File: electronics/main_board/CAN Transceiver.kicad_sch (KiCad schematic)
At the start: 2 parts, among them U18 TJA1051TK/3

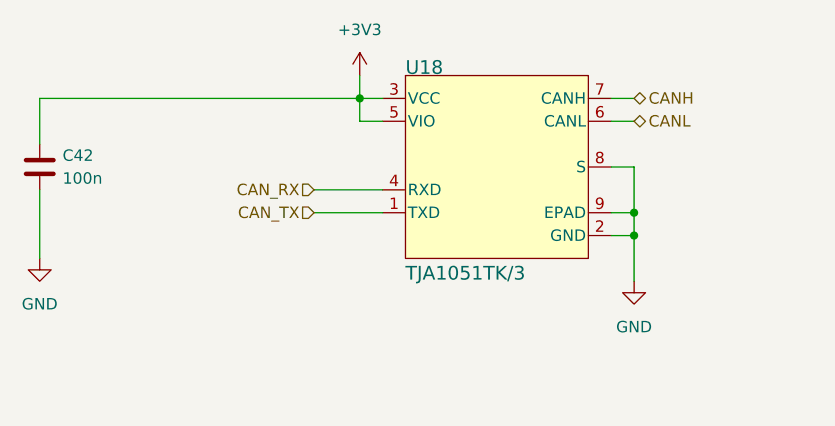
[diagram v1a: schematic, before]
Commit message: fix
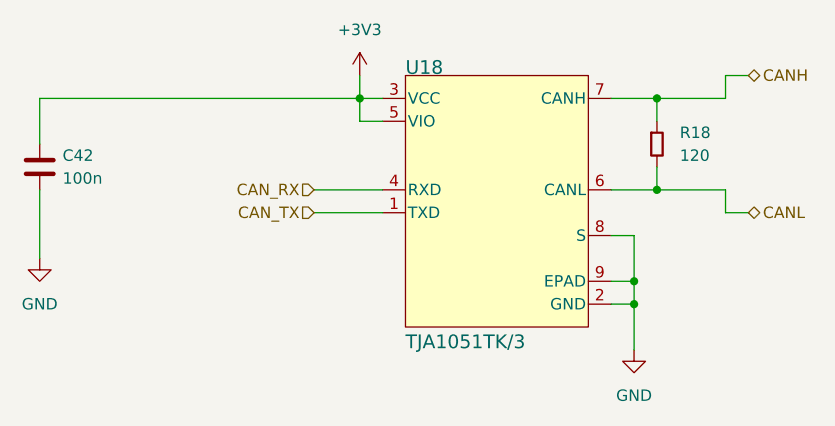
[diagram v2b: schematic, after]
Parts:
- added R18: 120, Resistor_SMD:R_0402_1005Metric, symbol Device:R
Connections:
- net CANH: now also R18.1
- net CANL: now also R18.2
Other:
- moved on the sheet: U18
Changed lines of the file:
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@@
 	(paper "A4")
 	(junction
-		(at 167.64 99.06)
+		(at 167.64 106.68)
+		(diameter 0)
+		(color 0 0 0 0)
+	)
+	(junction
+		(at 170.18 93.98)
 		(diameter 0)
 		(color 0 0 0 0)
@@
 	)
 	(junction
-		(at 167.64 96.52)
+		(at 170.18 83.82)
 		(diameter 0)
 		(color 0 0 0 0)
 	)
+	(junction
+		(at 167.64 104.14)
+		(diameter 0)
+		(color 0 0 0 0)
+	)
+	(wire
+		(pts
+			(xy 170.18 83.82) (xy 170.18 86.36)
+		)
+		(stroke
+			(width 0)
+			(type default)
+		)
+	)
 	(wire
 		(pts
@@
 	(wire
 		(pts
-			(xy 167.64 96.52) (xy 167.64 99.06)
+			(xy 177.8 81.28) (xy 177.8 83.82)
+		)
+		(stroke
+			(width 0)
+			(type default)
+		)
+	)
+	(wire
+		(pts
+			(xy 167.64 104.14) (xy 167.64 106.68)
 		)
 		(stroke
@@
 	(wire
 		(pts
+			(xy 165.1 93.98) (xy 170.18 93.98)
+		)
+		(stroke
+			(width 0)
+			(type default)
+		)
+	)
+	(wire
+		(pts
 			(xy 132.08 96.52) (xy 139.7 96.52)
 		)
@@
 	(wire
 		(pts
+			(xy 165.1 106.68) (xy 167.64 106.68)
+		)
+		(stroke
+			(width 0)
+			(type default)
+		)
+	)
+	(wire
+		(pts
+			(xy 177.8 96.52) (xy 177.8 93.98)
+		)
+		(stroke
+			(width 0)
+			(type default)
+		)
+	)
+	(wire
+		(pts
+			(xy 101.6 83.82) (xy 137.16 83.82)
+		)
+		(stroke
+			(width 0)
+			(type default)
+		)
+	)
+	(wire
+		(pts
+			(xy 101.6 83.82) (xy 101.6 88.9)
+		)
+		(stroke
+			(width 0)
+			(type default)
+		)
+	)
+	(wire
+		(pts
 			(xy 165.1 99.06) (xy 167.64 99.06)
 		)
@@
 	(wire
 		(pts
-			(xy 101.6 83.82) (xy 137.16 83.82)
-		)
-		(stroke
-			(width 0)
-			(type default)
-		)
-	)
-	(wire
-		(pts
-			(xy 101.6 83.82) (xy 101.6 88.9)
-		)
-		(stroke
-			(width 0)
-			(type default)
-		)
-	)
-	(wire
-		(pts
-			(xy 165.1 91.44) (xy 167.64 91.44)
+			(xy 170.18 93.98) (xy 177.8 93.98)
 		)
 		(stroke
@@
 	(wire
 		(pts
-			(xy 165.1 86.36) (xy 167.64 86.36)
-		)
-		(stroke
-			(width 0)
-			(type default)
-		)
-	)
-	(wire
-		(pts
-			(xy 165.1 96.52) (xy 167.64 96.52)
-		)
-		(stroke
-			(width 0)
-			(type default)
-		)
-	)
-	(wire
-		(pts
-			(xy 165.1 83.82) (xy 167.64 83.82)
-		)
-		(stroke
-			(width 0)
-			(type default)
-		)
-	)
-	(wire
-		(pts
-			(xy 167.64 96.52) (xy 167.64 91.44)
-		)
-		(stroke
-			(width 0)
-			(type default)
-		)
-	)
-	(wire
-		(pts
-			(xy 167.64 99.06) (xy 167.64 104.14)
+			(xy 170.18 91.44) (xy 170.18 93.98)
+		)
+		(stroke
+			(width 0)
+			(type default)
+		)
+	)
+	(wire
+		(pts
+			(xy 177.8 96.52) (xy 180.34 96.52)
+		)
+		(stroke
+			(width 0)
+			(type default)
+		)
+	)
+	(wire
+		(pts
+			(xy 165.1 104.14) (xy 167.64 104.14)
+		)
+		(stroke
+			(width 0)
+			(type default)
+		)
+	)
+	(wire
+		(pts
+			(xy 177.8 81.28) (xy 180.34 81.28)
+		)
+		(stroke
+			(width 0)
+			(type default)
+		)
+	)
+	(wire
+		(pts
+			(xy 167.64 104.14) (xy 167.64 99.06)
+		)
+		(stroke
+			(width 0)
+			(type default)
+		)
+	)
+	(wire
+		(pts
+			(xy 167.64 106.68) (xy 167.64 111.76)
+		)
+		(stroke
+			(width 0)
+			(type default)
+		)
+	)
+	(wire
+		(pts
+			(xy 170.18 83.82) (xy 177.8 83.82)
+		)
+		(stroke
+			(width 0)
+			(type default)
+		)
+	)
+	(wire
+		(pts
+			(xy 165.1 83.82) (xy 170.18 83.82)
 		)
 		(stroke
@@
 	(hierarchical_label "CANL"
 		(shape bidirectional)
-		(at 167.64 86.36 0)
+		(at 180.34 96.52 0)
 		(effects
 			(font
@@
 	(hierarchical_label "CANH"
 		(shape bidirectional)
-		(at 167.64 83.82 0)
+		(at 180.34 81.28 0)
 		(effects
 			(font
@@
 	(symbol
 		(lib_id "power:GND")
-		(at 167.64 104.14 0)
+		(at 167.64 111.76 0)
 		(unit 1)
 		(exclude_from_sim no)
@@
 		(fields_autoplaced yes)
 		(property "Reference" "#PWR0119"
-			(at 167.64 110.49 0)
+			(at 167.64 118.11 0)
 			(effects
 				(font
@@
 		)
 		(property "Value" "GND"
-			(at 167.64 109.22 0)
+			(at 167.64 116.84 0)
 			(effects
 				(font
@@
 		)
 		(property "Footprint" ""
-			(at 167.64 104.14 0)
+			(at 167.64 111.76 0)
 			(effects
 				(font
@@
 		)
 		(property "Datasheet" ""
-			(at 167.64 104.14 0)
+			(at 167.64 111.76 0)
 			(effects
 				(font
@@
 		)
 		(property "Description" "Power symbol creates a global label with name \"GND\" , ground"
-			(at 167.64 104.14 0)
+			(at 167.64 111.76 0)
 			(effects
 				(font
@@
 		)
 		(property "Value" "TJA1051TK/3"
-			(at 142.24 104.14 0)
+			(at 142.24 111.76 0)
 			(effects
 				(font
@@
 					(unit 1)
 				)
+			)
+		)
+	)
+	(symbol
+		(lib_id "Device:R")
+		(at 170.18 88.9 0)
+		(unit 1)
+		(exclude_from_sim no)
+		(in_bom yes)
+		(on_board yes)
+		(dnp no)
+		(fields_autoplaced yes)
+		(property "Reference" "R18"
+			(at 172.72 87.6299 0)
+			(effects
+				(font
+					(size 1.27 1.27)
+				)
+				(justify left)
+			)
+		)
+		(property "Value" "120"
+			(at 172.72 90.1699 0)
+			(effects
+				(font
+					(size 1.27 1.27)
+				)
+				(justify left)
+			)
+		)
+		(property "Footprint" "Resistor_SMD:R_0402_1005Metric"
+			(at 168.402 88.9 90)
+			(effects
+				(font
+					(size 1.27 1.27)
+				)
+				(hide yes)
+			)
+		)
+		(property "Datasheet" "~"
+			(at 170.18 88.9 0)
+			(effects
+				(font
+					(size 1.27 1.27)
+				)
+				(hide yes)
+			)
+		)
+		(property "Description" "Resistor"
+			(at 170.18 88.9 0)
+			(effects
+				(font
+					(size 1.27 1.27)
+				)
+				(hide yes)
+			)
+		)
+		(property "Manufacturer" "Vishay Intertech"
+			(at 170.18 88.9 0)
+			(effects
+				(font
+					(size 1.27 1.27)
+				)
+				(hide yes)
+			)
+		)
+		(property "Manufacturer Part Number" "CRCW0603120RFKEAHP"
+			(at 170.18 88.9 0)
+			(effects
+				(font
+					(size 1.27 1.27)
+				)
+				(hide yes)
+			)
+		)
+		(pin "1"
+		)
+		(pin "2"
+		)
+		(instances
+			(project "main_board"
+				(path "/82f7d8d0-a6dd-48aa-80fa-49fc2cccb16f/1b9d8d50-bf31-43c5-a329-47671a272977"
+					(reference "R18")
+					(unit 1)
+				)
+				(path "/82f7d8d0-a6dd-48aa-80fa-49fc2cccb16f/51a0530e-a541-446c-8cbb-8049bd9a895b"
+					(reference "R19")
+					(unit 1)
+				)
